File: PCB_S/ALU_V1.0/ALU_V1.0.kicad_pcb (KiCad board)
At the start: 6 copper layers, 115 x 100 mm, 528 parts, among them J1 Conn_01x08_Socket, J2 Conn_01x08_Socket, J3 Conn_01x08_Socket, J8 Conn_01x14_Pin, Q1 2N7002, Q10 2N7002, Q100 2N7002, Q101 2N7002, Q102 2N7002, Q103 2N7002, Q104 2N7002, Q105 2N7002, Q106 2N7002, Q107 2N7002, Q108 2N7002, Q109 2N7002, Q11 2N7002, Q110 2N7002, Q111 2N7002, Q112 2N7002, Q113 2N7002, Q114 2N7002, Q115 2N7002, Q116 2N7002, Q117 2N7002, Q118 2N7002, Q119 2N7002, Q12 2N7002, Q120 2N7002, Q121 2N7002, Q122 2N7002, Q123 2N7002, Q124 2N7002, Q125 2N7002, Q126 2N7002, Q127 2N7002, Q128 2N7002, Q129 2N7002, Q13 2N7002, Q130 2N7002, Q131 2N7002, Q132 2N7002, Q133 2N7002, Q134 2N7002, Q135 2N7002, Q136 2N7002, Q137 2N7002, Q138 2N7002, Q139 2N7002, Q14 2N7002, Q140 2N7002, Q141 2N7002, Q142 2N7002, Q143 2N7002, Q144 2N7002, Q145 2N7002, Q146 2N7002, Q147 2N7002, Q148 2N7002, Q149 2N7002, Q15 2N7002, Q150 2N7002, Q151 2N7002, Q152 2N7002, Q153 2N7002, Q154 2N7002, Q155 2N7002, Q156 2N7002, Q157 2N7002, Q158 2N7002, Q159 2N7002, Q16 2N7002, Q160 2N7002, Q161 2N7002, Q162 2N7002, Q163 2N7002, Q164 2N7002, Q165 2N7002, Q166 2N7002, Q167 2N7002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

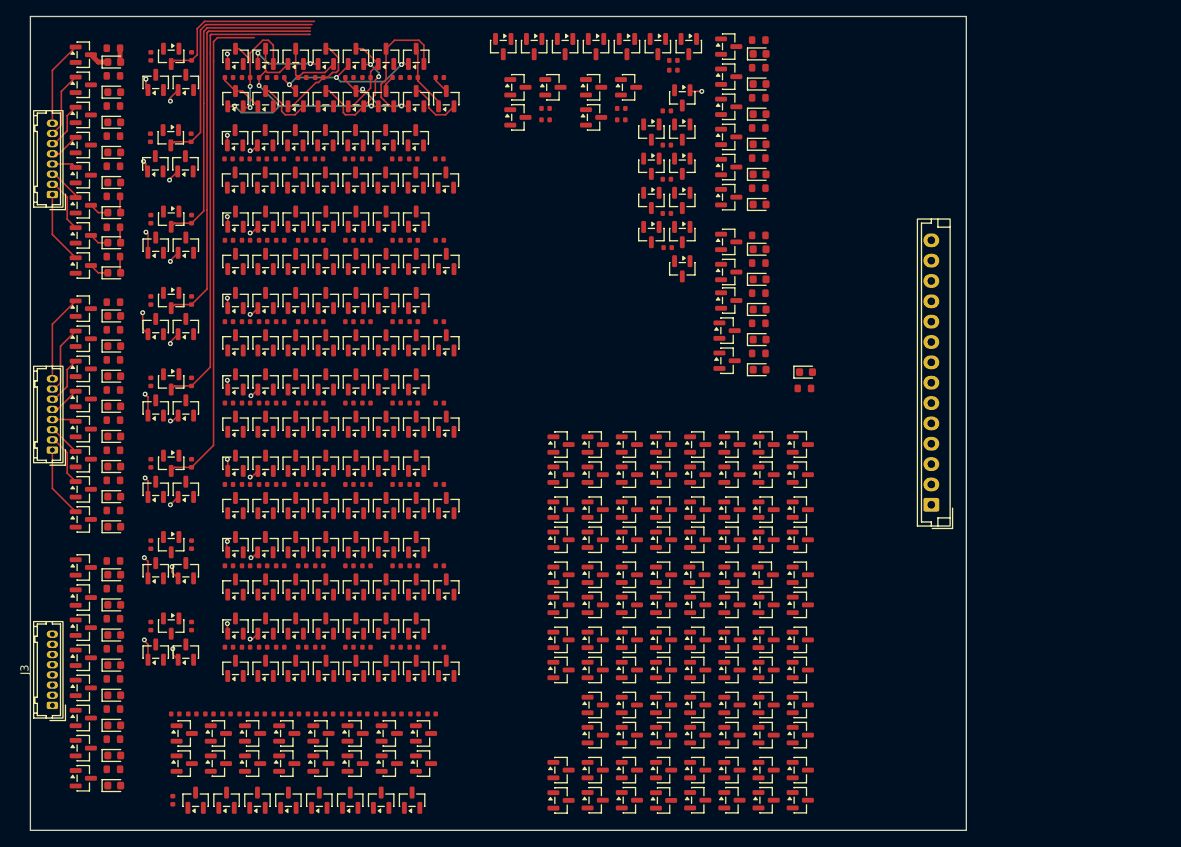
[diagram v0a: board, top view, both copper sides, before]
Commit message: ALU_V1.0 WIP
making pcb
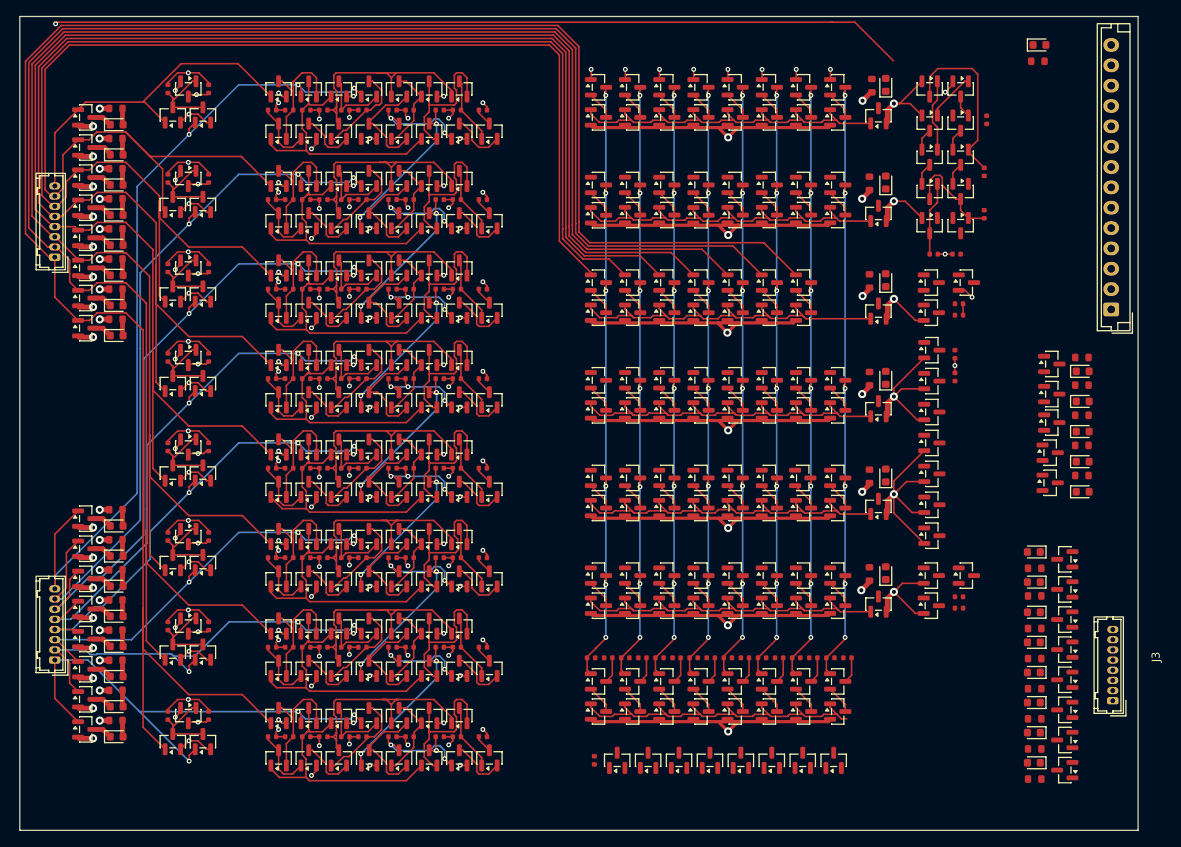
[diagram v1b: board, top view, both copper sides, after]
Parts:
- moved J3 130.3 mm to (178.2, 111.1)
- moved Q273 120.7 mm to (172.3, 93.7), turned to 180 degrees
- moved Q272 120.6 mm to (172.3, 97.4), turned to 180 degrees
- moved Q274 120.6 mm to (172.3, 101.1), turned to 180 degrees
- moved Q275 120.6 mm to (172.3, 104.8), turned to 180 degrees
- moved Q276 120.6 mm to (172.3, 108.5), turned to 180 degrees
- moved Q291 120.6 mm to (172.3, 112.2), turned to 180 degrees
- moved Q292 120.6 mm to (172.3, 115.9), turned to 180 degrees
- moved Q293 120.6 mm to (172.3, 119.6), turned to 180 degrees
- moved R128 113.3 mm to (168.6, 98.2), turned to 180 degrees
- moved R134 113.2 mm to (168.6, 94.8), turned to 180 degrees
- moved R135 113.2 mm to (168.6, 102.2), turned to 180 degrees
- moved R136 113.2 mm to (168.6, 105.9), turned to 180 degrees
- moved R137 113.2 mm to (168.6, 109.6), turned to 180 degrees
- moved R138 113.2 mm to (168.6, 113.3), turned to 180 degrees
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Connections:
- D36 pad 1: Earth -> GND
- J8 pad 13: Earth -> GND
- Q272 pad 2: Earth -> GND
- Q273 pad 2: Earth -> GND
- Q274 pad 2: Earth -> GND
- Q275 pad 2: Earth -> GND
- Q276 pad 2: Earth -> GND
- Q291 pad 2: Earth -> GND
- Q292 pad 2: Earth -> GND
- Q293 pad 2: Earth -> GND
- Q294 pad 2: Earth -> GND
- Q295 pad 2: Earth -> GND
- Q296 pad 2: Earth -> GND
- Q297 pad 2: Earth -> GND
- Q298 pad 2: Earth -> GND
- Q299 pad 2: Earth -> GND
- Q300 pad 2: Earth -> GND
- Q301 pad 2: Earth -> GND
- Q302 pad 2: Earth -> GND
- Q303 pad 2: Earth -> GND
- Q304 pad 2: Earth -> GND
- Q305 pad 2: Earth -> GND
- Q306 pad 2: Earth -> GND
- Q307 pad 2: Earth -> GND
- Q308 pad 2: Earth -> GND
- Q309 pad 2: Earth -> GND
- Q310 pad 2: Earth -> GND
- Q311 pad 2: Earth -> GND
- Q312 pad 2: Earth -> GND
- Q313 pad 2: Earth -> GND
- Q314 pad 2: Earth -> GND
- Q315 pad 2: Earth -> GND
- Q316 pad 2: Earth -> GND
- Q317 pad 2: Earth -> GND
- Q318 pad 2: Earth -> GND
- Q319 pad 2: Earth -> GND
- Q320 pad 2: Earth -> GND
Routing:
- net GND: track 0.00 -> 440.0 mm, vias 0 -> 95
- net Net-(Q147-G): track 0.00 -> 189.4 mm, vias 0 -> 2
- net VCC: track 0.00 -> 184.6 mm, vias 0 -> 80
- net Net-(J1-Pin_1): track 83.8 -> 256.1 mm, vias 2 -> 0
- net Net-(Q148-G): track 0.00 -> 167.8 mm, vias 0 -> 2
- net Net-(J1-Pin_2): track 73.1 -> 231.2 mm, vias 2 -> 0
- net Net-(J1-Pin_3): track 62.0 -> 214.8 mm, vias 2 -> 0
- net Net-(J1-Pin_4): track 52.3 -> 201.1 mm, vias 2 -> 0
- net Net-(J1-Pin_5): track 44.3 -> 187.5 mm, vias 2 -> 0
- net Net-(J1-Pin_6): track 37.2 -> 169.5 mm, vias 2 -> 0
- net Net-(J1-Pin_7): track 35.1 -> 158.1 mm, vias 2 -> 0
- net Net-(J1-Pin_8): track 46.3 -> 167.1 mm, vias 2 -> 1
- net Net-(Q149-G): track 61.3 -> 151.6 mm, vias 0 -> 2
- net Net-(Q150-D): track 0.00 -> 81.5 mm, vias 0 -> 7
- net Net-(Q152-D): track 0.00 -> 81.3 mm, vias 0 -> 7
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- added copper zone on In3.Cu, net GND
- added copper zone on In2.Cu, net VCC
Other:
- board size 115 x 100 mm -> 137.4 x 100 mm
- board text removed: "${REFERENCE}"
